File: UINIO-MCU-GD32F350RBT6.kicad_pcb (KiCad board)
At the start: 2 copper layers, 88.1 x 20.3 mm, 37 parts, among them J1 Conn_01x32_Pin, J2 Conn_01x32_Pin, J3 Conn_01x04_Pin, SW1 BOOT0, SW2 NRST, U1 ME6211C33M5G-N, U2 GD32F350RBT6, Y1 32.768KHz, Y2 8MHz

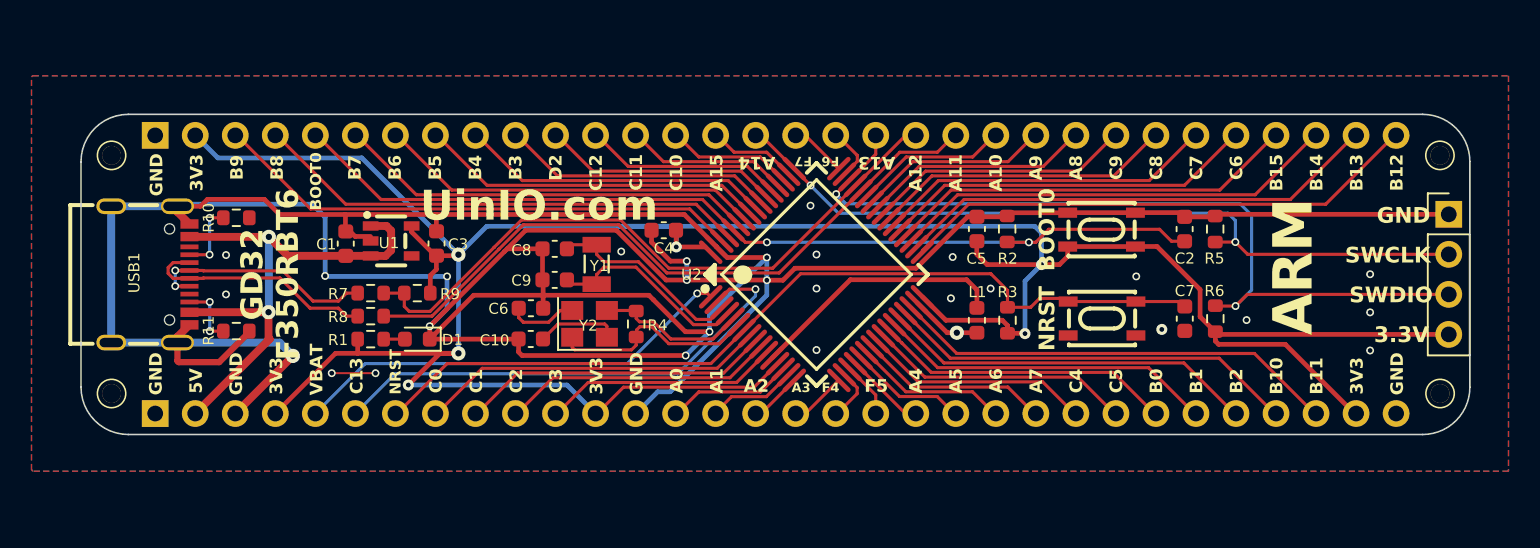
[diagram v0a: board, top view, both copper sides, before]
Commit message: Release UINIO-MCU-GD32F350RBT6 version 3.2.0.
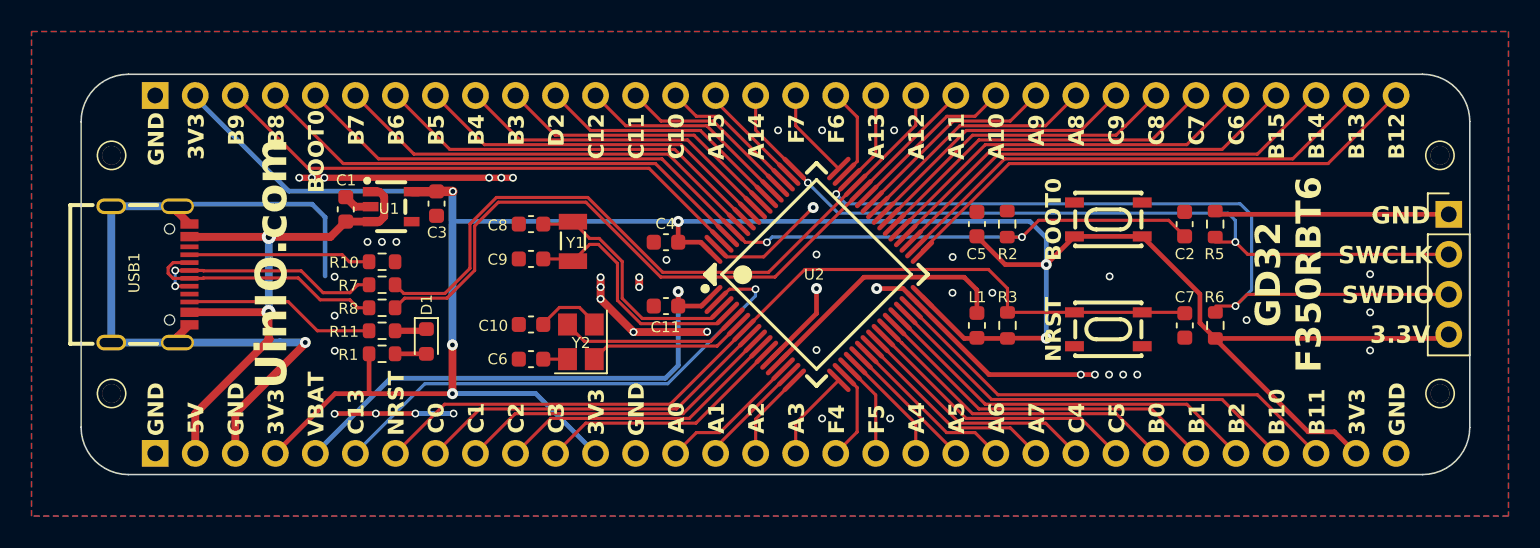
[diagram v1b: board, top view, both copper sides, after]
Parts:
- removed R4: 1M, Resistor_SMD:R_0603_1608Metric
- removed R9: 1.5K, Resistor_SMD:R_0603_1608Metric
- added C11: 0.1uF, Capacitor_SMD:C_0603_1608Metric, F.Cu at (143.5, 105.6)
- moved R10 9.66 mm to (125.5, 102.8)
- moved R11 9.25 mm to (125.5, 107.2)
- moved C6 3.23 mm to (134.9, 109.0), turned to 0 degrees
- moved C3 2.53 mm to (128.9, 99.1), turned to 90 degrees
- moved J1 2.53 mm to (111.1, 115.0)
- moved J2 2.53 mm to (111.1, 92.3)
- moved C1 2.18 mm to (123.2, 99.5)
- moved U1 2.18 mm to (126.1, 99.3)
- moved C8 2.17 mm to (134.9, 100.4)
- moved Y1 2.10 mm to (137.6, 101.5)
- moved C9 2.01 mm to (134.9, 102.7)
- moved Y2 1.27 mm to (138.1, 107.9), turned to 90 degrees
- moved R1 1.18 mm to (125.5, 108.7)
- moved C10 0.92 mm to (134.9, 106.8)
- moved R8 0.90 mm to (125.5, 105.8)
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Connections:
- L1 pad 1: GND -> /VDD_3.3V
- L1 pad 2: /VSSA -> Net-(U2-VDDA)
- U2 pad 12: /VSSA -> GND
- U2 pad 13: /VDD_3.3V -> Net-(U2-VDDA)
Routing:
- net GND: track 254.8 -> 129.0 mm, vias 29 -> 48
- net /VDD_3.3V: track 185.6 -> 166.4 mm
- net /VSSA: track 16.5 -> 0.00 mm
- net Net-(U2-VDDA): track 0.00 -> 16.1 mm
- net Net-(USB1-CC2): track 4.00 -> 12.1 mm, vias 2 -> 0
- net Net-(USB1-CC1): track 4.49 -> 11.6 mm, vias 2 -> 0
- net /VBAT: track 28.3 -> 33.2 mm
- net /PA12: track 41.4 -> 45.2 mm
- net /PF1: track 13.3 -> 10.1 mm
- net Net-(U2-PC14-OSC32IN): track 12.2 -> 15.4 mm
- net Net-(U2-PC15-OSC32OUT): track 12.5 -> 15.7 mm
- net /PA11: track 43.6 -> 46.7 mm
- net Net-(C6-Pad2): track 4.42 -> 1.54 mm
- net /PA4: track 4.47 -> 7.28 mm
- net /PA2: track 2.97 -> 5.64 mm
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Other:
- board size 88.1 x 20.3 mm -> 88.1 x 25.4 mm
- board text added: "Version 3.2.0"
- board text removed: "ARM"
- board text removed: "Version 3.1.1"
